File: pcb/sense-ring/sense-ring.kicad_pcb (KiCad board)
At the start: 2 copper layers, 78 x 68.6 mm, 53 parts, among them J1 Conn_ARM_SWD_TagConnect_TC203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, J2 Conn_01x04_MountingPin, J3 Conn_01x04_MountingPin, U1 TJA1044GTK/3, U10 STM32G431KBUx, U11 NCP176, U2 LPS22HH, U3 LPS22HH, U4 LPS22HH, U5 LPS22HH, U6 LPS22HH, U7 LPS22HH, U8 LPS22HH, U9 ICM-42688-P, Y1 16MHz

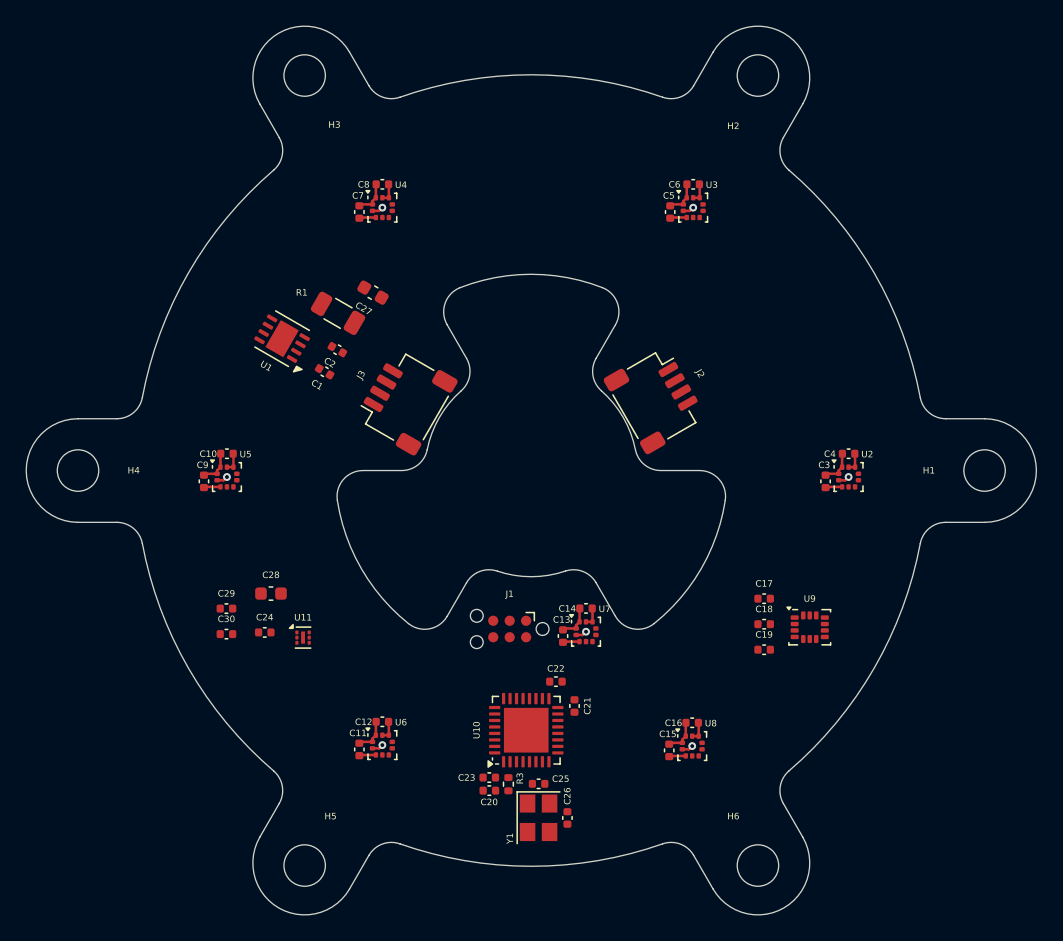
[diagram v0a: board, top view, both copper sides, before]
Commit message: Finish sense-ring
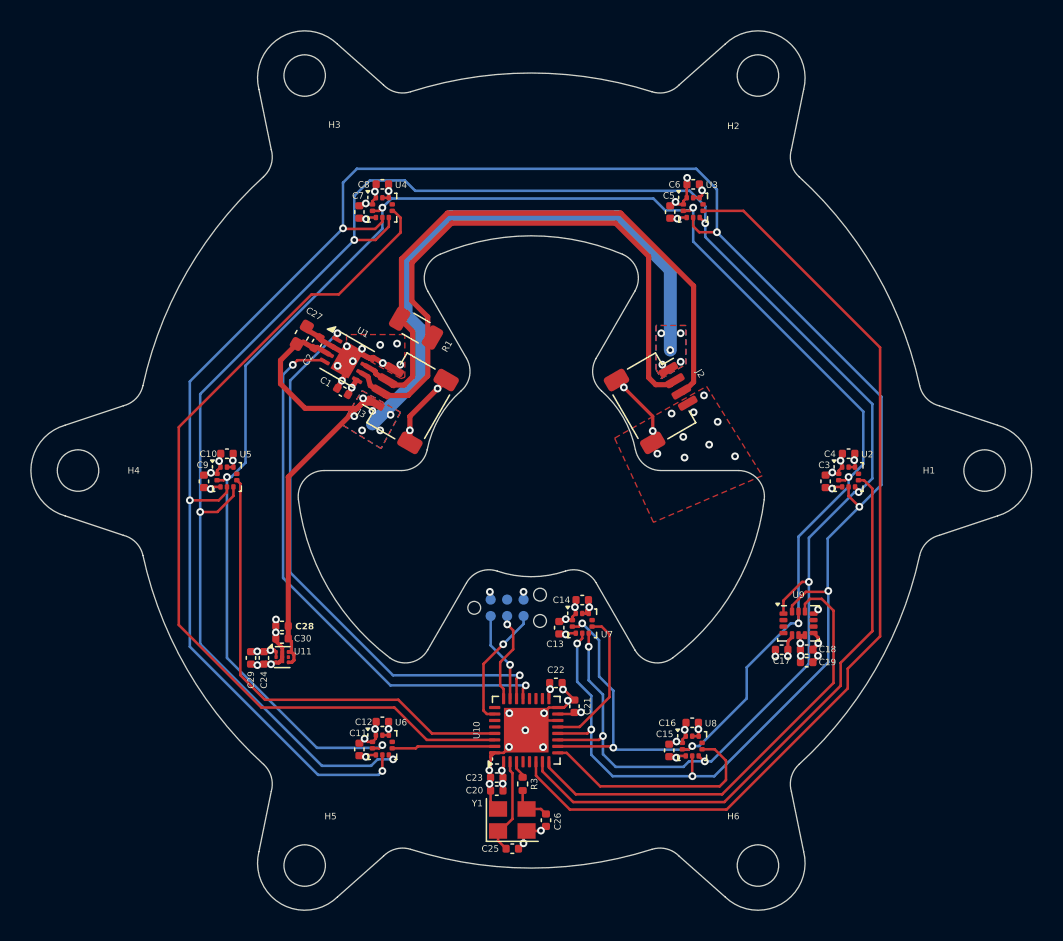
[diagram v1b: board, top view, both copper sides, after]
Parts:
- C17: value 10n -> 100n
- C28: footprint Capacitor_SMD:C_0603_1608Metric -> Capacitor_SMD:C_0402_1005Metric
- J1: moved to B.Cu
- moved C27 6.40 mm to (94.3, 94.6), turned to 60 degrees
- moved R1 6.13 mm to (103.1, 94.0)
- moved C25 5.40 mm to (110.5, 134.2)
- moved U1 5.28 mm to (97.8, 96.5), turned to -30 degrees
- moved C30 4.31 mm to (92.8, 118.0), turned to 180 degrees
- moved C29 4.25 mm to (90.4, 119.5), turned to -90 degrees
- moved C17 4.17 mm to (131.3, 118.8), turned to 180 degrees
- moved C18 3.82 mm to (133.3, 118.8), turned to 180 degrees
- moved C19 3.42 mm to (133.3, 119.8), turned to 180 degrees
- moved C28 2.64 mm to (92.8, 117.0), turned to 180 degrees
- moved U11 2.20 mm to (92.8, 119.4)
- moved C1 2.07 mm to (97.4, 98.9)
- moved Y1 2.03 mm to (110.5, 132.0), turned to 0 degrees
- moved C24 1.97 mm to (91.4, 119.5), turned to -90 degrees
- moved C26 1.67 mm to (113.1, 132.0), turned to 90 degrees
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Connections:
- C25 pad 2: /XTALO -> /XTALI
- J1 pad 3: /RST -> unconnected-(J1-~{RESET}-Pad3)
- R3 pad 2: /XTALI -> /XTALO
- U10 pad 13: unconnected-(U10-PB0-Pad13) -> /CS7
- U10 pad 21: unconnected-(U10-PA11-Pad21) -> /CNRX
- U10 pad 22: unconnected-(U10-PA12-Pad22) -> /CNTX
- U10 pad 29: unconnected-(U10-PB6-Pad29) -> /CS4
- U10 pad 30: unconnected-(U10-PB7-Pad30) -> /CS3
- U10 pad 31: unconnected-(U10-PB8-Pad31) -> /CS5
- U10 pad 6: unconnected-(U10-PA1-Pad6) -> /CS2
- U10 pad 7: unconnected-(U10-PA2-Pad7) -> /CS1
- U10 pad 8: unconnected-(U10-PA3-Pad8) -> /CS8
- U10 pad 9: unconnected-(U10-PA4-Pad9) -> /CS6
- Y1 pad 1: /XTALO -> /XTALI
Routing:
- net /MOSI: track 0.00 -> 186.9 mm, vias 0 -> 9
- net /MISO: track 0.00 -> 176.2 mm, vias 0 -> 9
- net /SCK: track 6.06 -> 161.0 mm, vias 7 -> 9
- net +5V: track 0.00 -> 82.1 mm, vias 0 -> 11
- net /CS2: track 0.00 -> 75.5 mm
- net /CS3: track 0.00 -> 68.7 mm
- net GND: track 19.9 -> 74.9 mm, vias 0 -> 56
- net /CANH: track 0.00 -> 48.9 mm
- net /CANL: track 0.00 -> 48.2 mm
- net /CS1: track 0.00 -> 46.0 mm
- net /CNTX: track 0.00 -> 43.4 mm, vias 0 -> 2
- net /CNRX: track 0.00 -> 42.7 mm, vias 0 -> 2
- net /CS4: track 0.00 -> 36.7 mm
- net /CS8: track 0.00 -> 35.7 mm
- net /CS6: track 0.00 -> 18.0 mm
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- added copper zone on In2.Cu, net +3V3
- added copper zone on B.Cu, net +5V
- added copper zone on F.Cu, net +5V
- added copper zone on F.Cu, net GND
- added copper zone on In1.Cu, net GND
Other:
- board size 78 x 68.6 mm -> 77.3 x 67.9 mm
- copper layers 2 -> 4
